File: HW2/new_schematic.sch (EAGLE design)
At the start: 2 parts

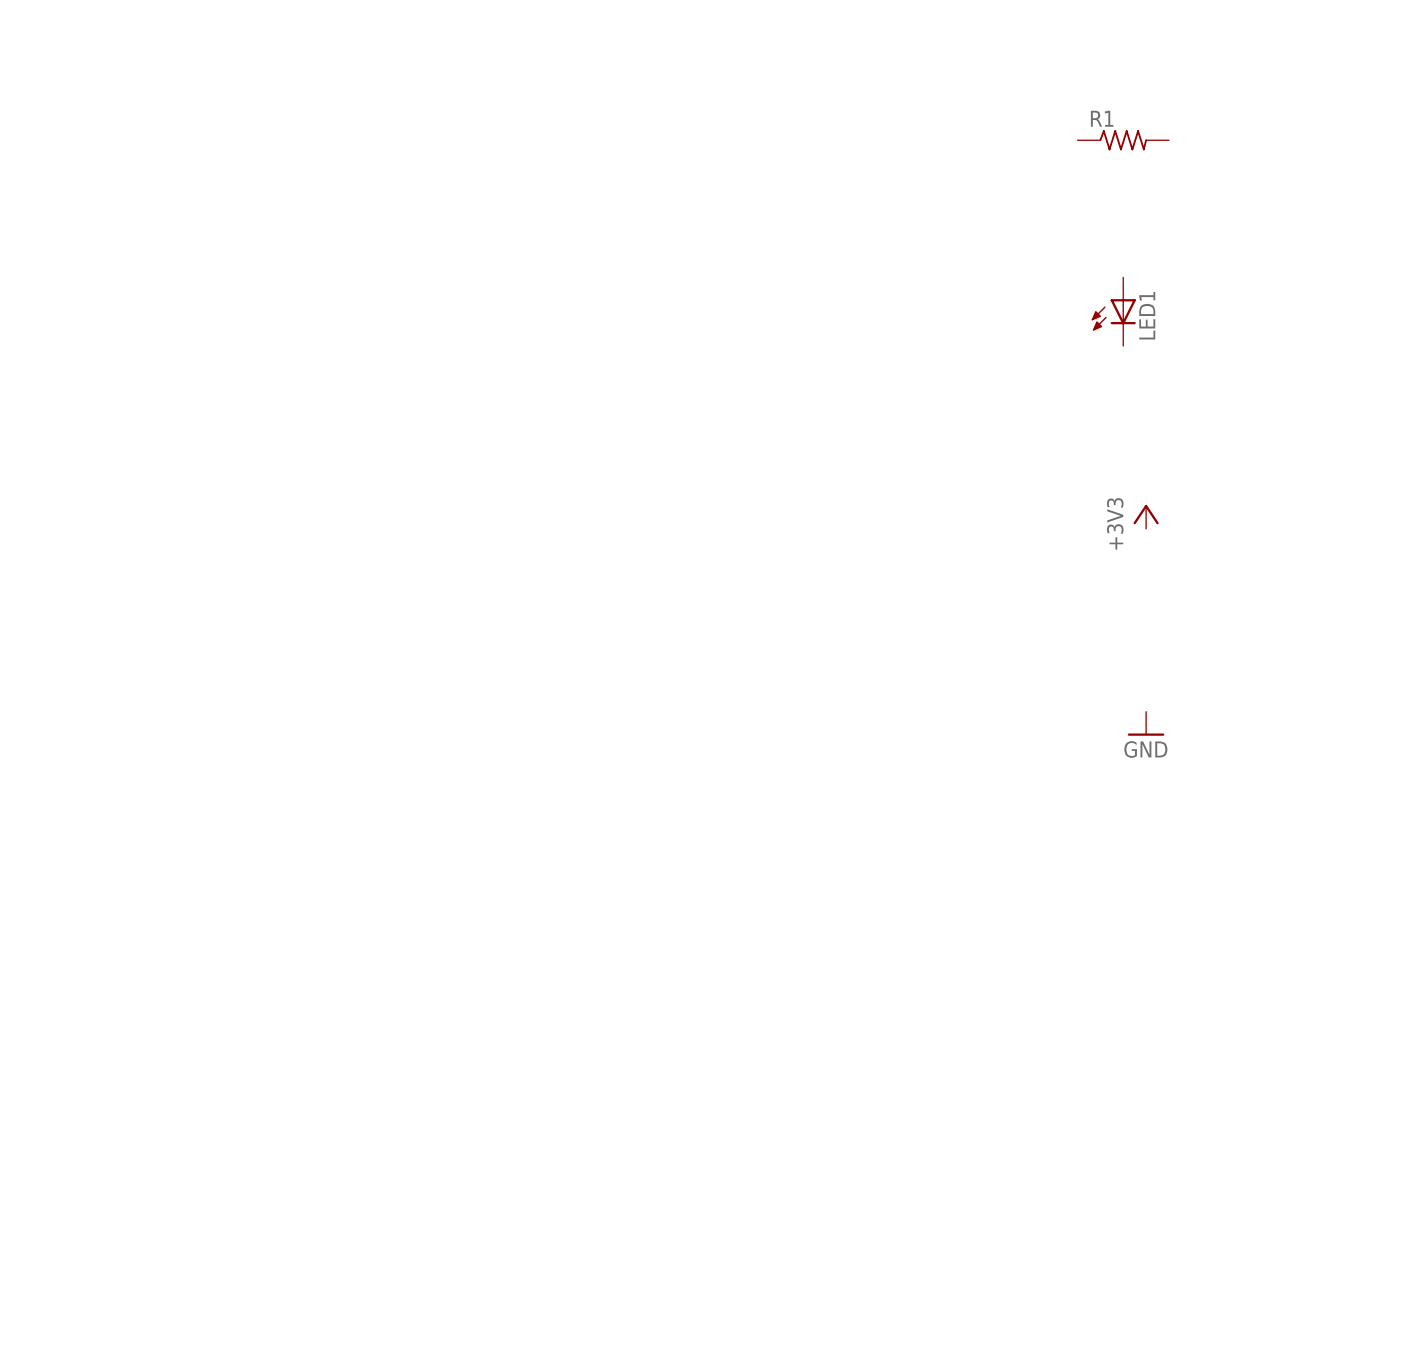
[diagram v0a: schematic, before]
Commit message: version_1
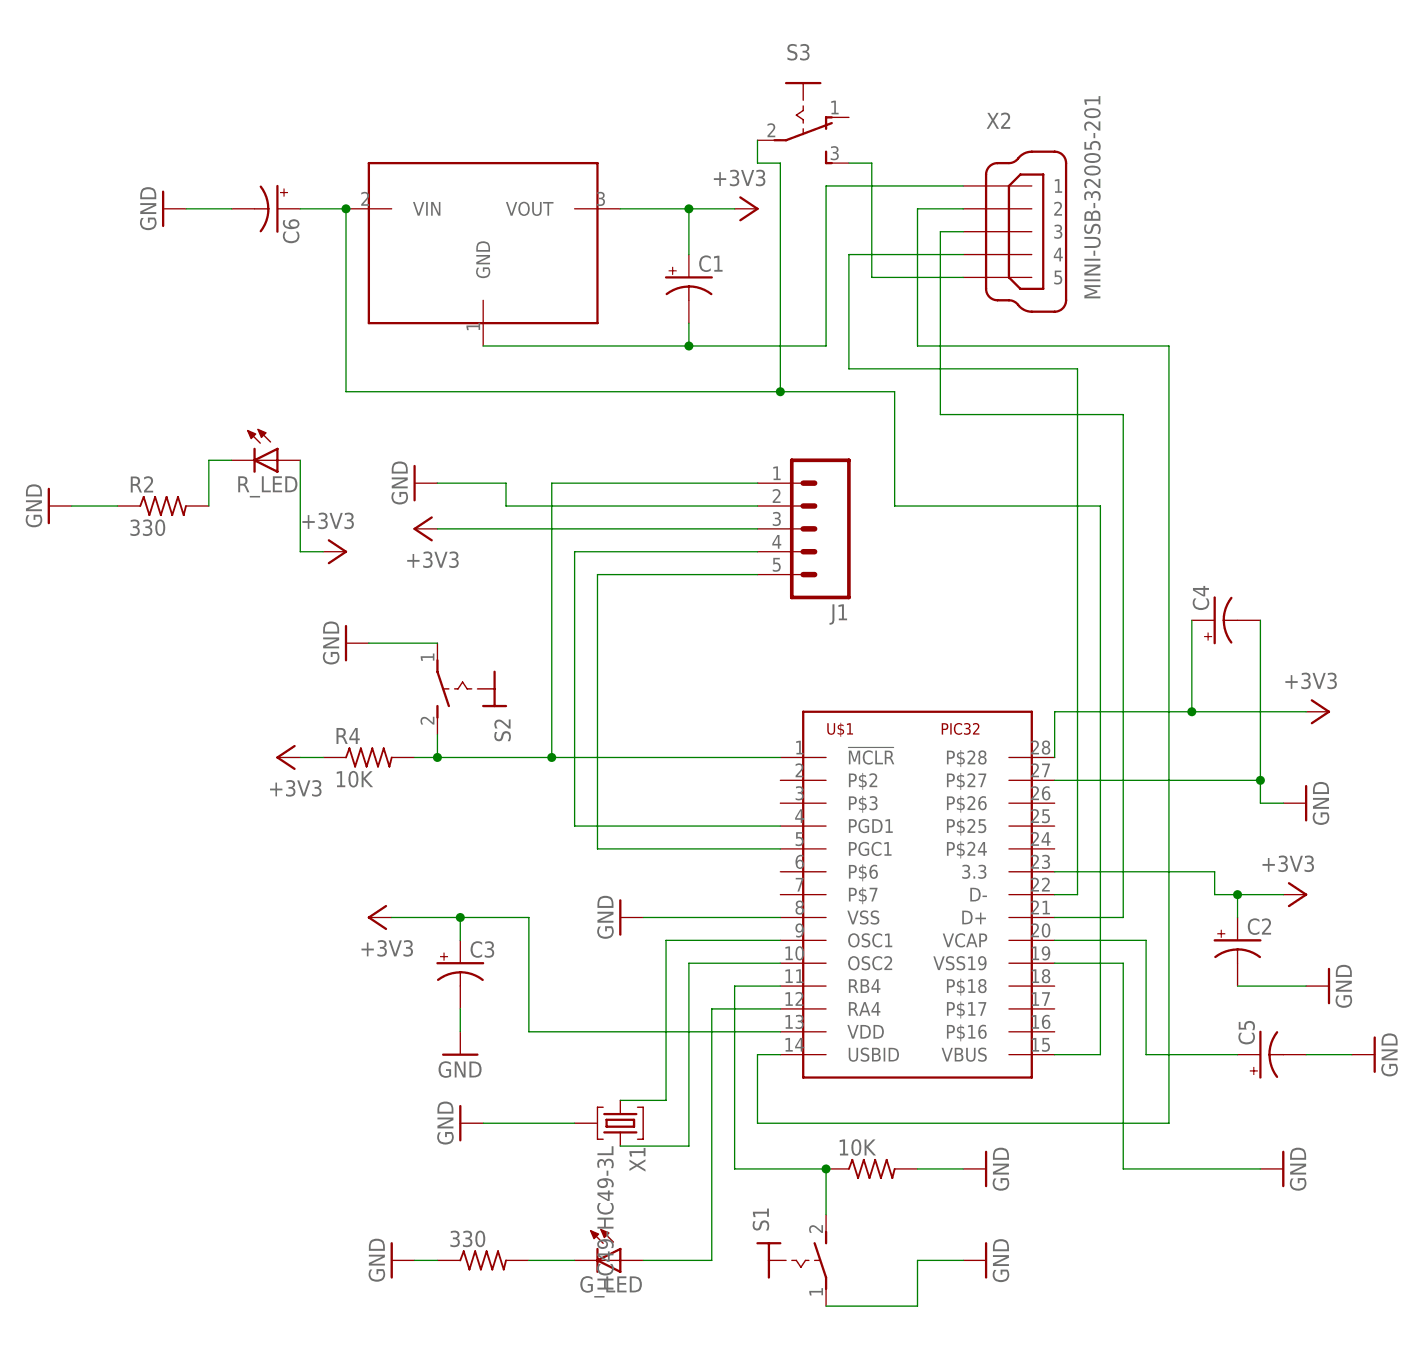
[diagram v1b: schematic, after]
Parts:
- removed LED1: (no value), led:LED3MM
- removed R1: (no value), resistor:R-US_0207/10
- added 10K, 330: (no value), new_library:R-US_0207/10
- added C1, C2, C3, C4, C5, C6: (no value), new_library:10UF-25V-20%(PTH)KIT
- added G_LED, R_LED: (no value), new_library:LED3MM
- added J1: (no value), new_library:M05NO_SILK
- added R2: 330, new_library:R-US_0207/10
- added R4: 10K, new_library:R-US_0207/10
- added S1, S2: (no value), new_library:MS243
- added S3: (no value), switch:M251
- added U$1: PIC32, new_library:PIC32
- added U$9: MCP1702, new_library:MCP1702
- added X1: HC49-HC49-3L, new_library:HC49-HC49-3L
- added X2: MINI-USB-32005-201, con-cypressindustries:MINI-USB-32005-201
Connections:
- new net +3V3: C1.+, C2.+, C3.+, C4.+, J1.3, R4.1, R_LED.A, U$1.3.3, U$1.P$28, U$1.VDD, U$9.VOUT
- new net GND: 10K.2, 330.1, C2.-, C3.-, C4.-, C5.-, C6.-, J1.2, R2.1, S1.P, S2.P, U$1.P$27, U$1.VSS, U$1.VSS19, X1.2
- new net N$1: U$1.USBID, X2.2
- new net N$10: C5.+, U$1.VCAP
- new net N$11: 330.2, G_LED.C
- new net N$12: G_LED.A, U$1.RA4
- new net N$13: S3.S, X2.5
- new net N$14: C6.+, S3.P, U$1.VBUS, U$9.VIN
- new net N$15: U$1.D-, X2.4
- new net N$16: U$1.D+, X2.3
- new net N$2: J1.4, U$1.PGD1
- new net N$3: J1.5, U$1.PGC1
- new net N$4: U$1.OSC1, X1.1
- new net N$5: U$1.OSC2, X1.3
- new net N$6: 10K.1, S1.S, U$1.RB4
- new net N$7: C1.-, U$9.GND, X2.1
- new net N$8: R2.2, R_LED.C
- new net N$9: J1.1, R4.2, S2.S, U$1.!MCLR
